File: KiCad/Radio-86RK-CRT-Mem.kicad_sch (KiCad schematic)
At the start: 20 parts, among them J1 Video, Q1 2N3904, U10 2716/КР573РФ5, U11 2716/КР573РФ5, U13 74198/К155ИР13, U15 7492/К155ИЕ4, U16 7486/К155ЛП5, U17 7474/К155ТМ2, U18 7408/К155ЛИ1, U19 7404/К155ЛН1, U8 8275/КР580ВГ75, U9 AS6C62256

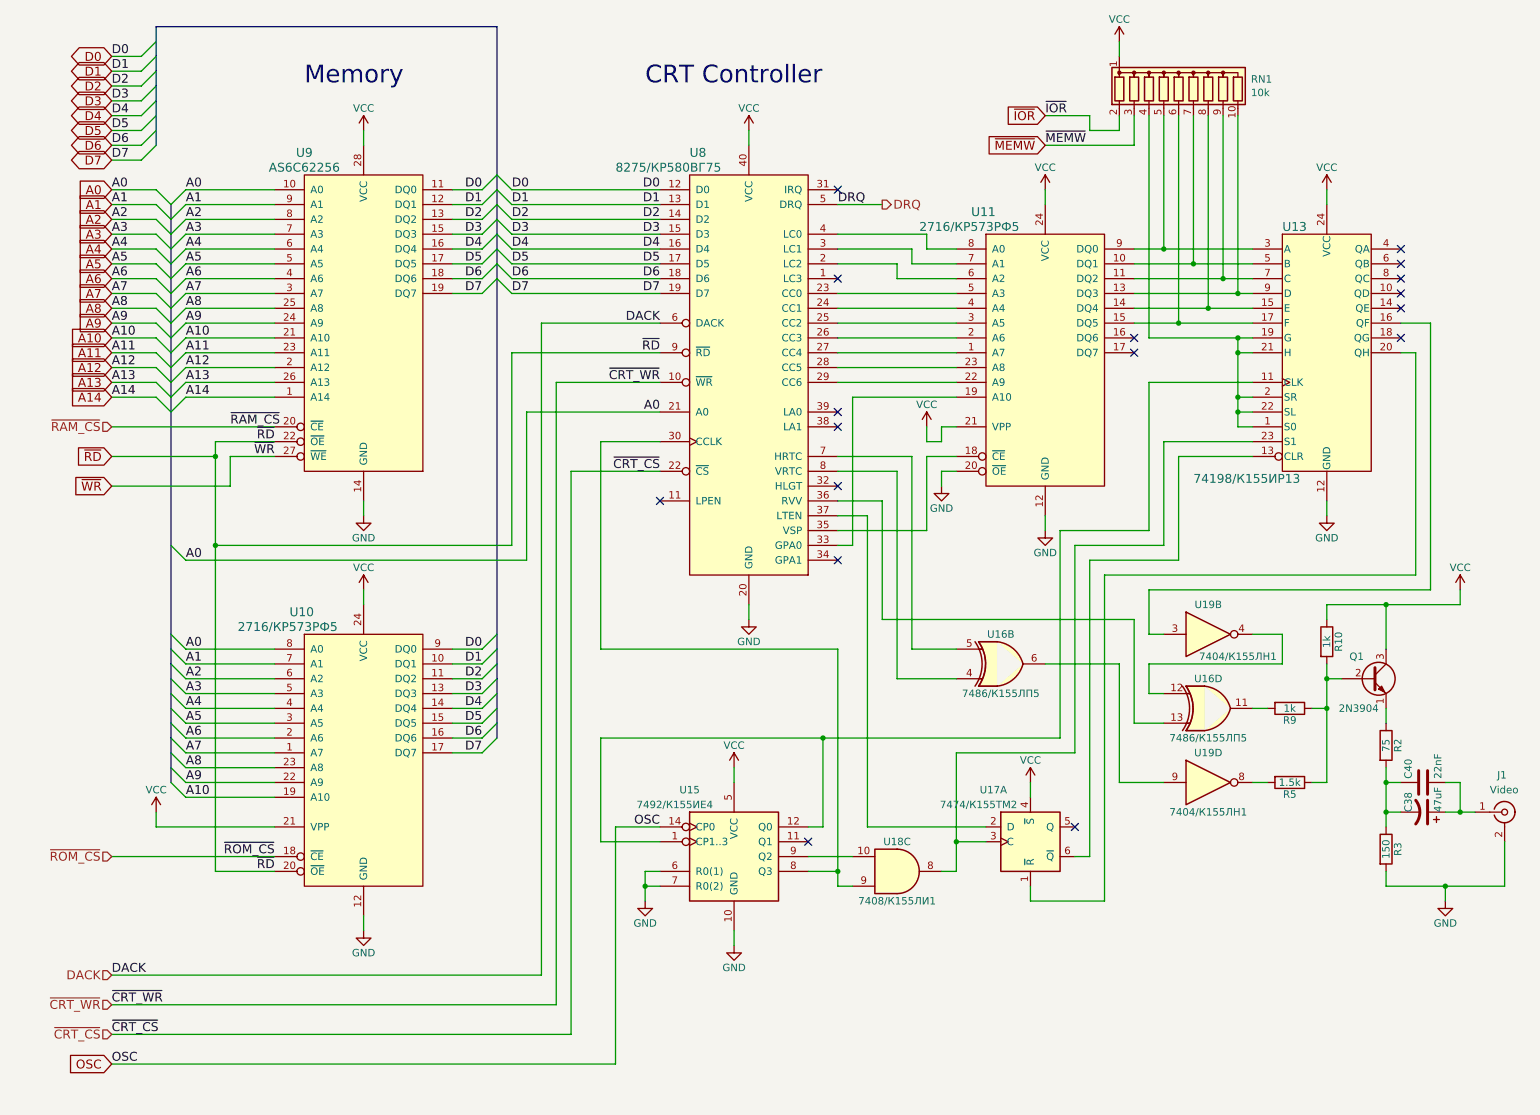
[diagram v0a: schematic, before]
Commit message: Add Version 1.4 files
Signed-off-by: Sergey Kiselev <skiselev@gmail.com>
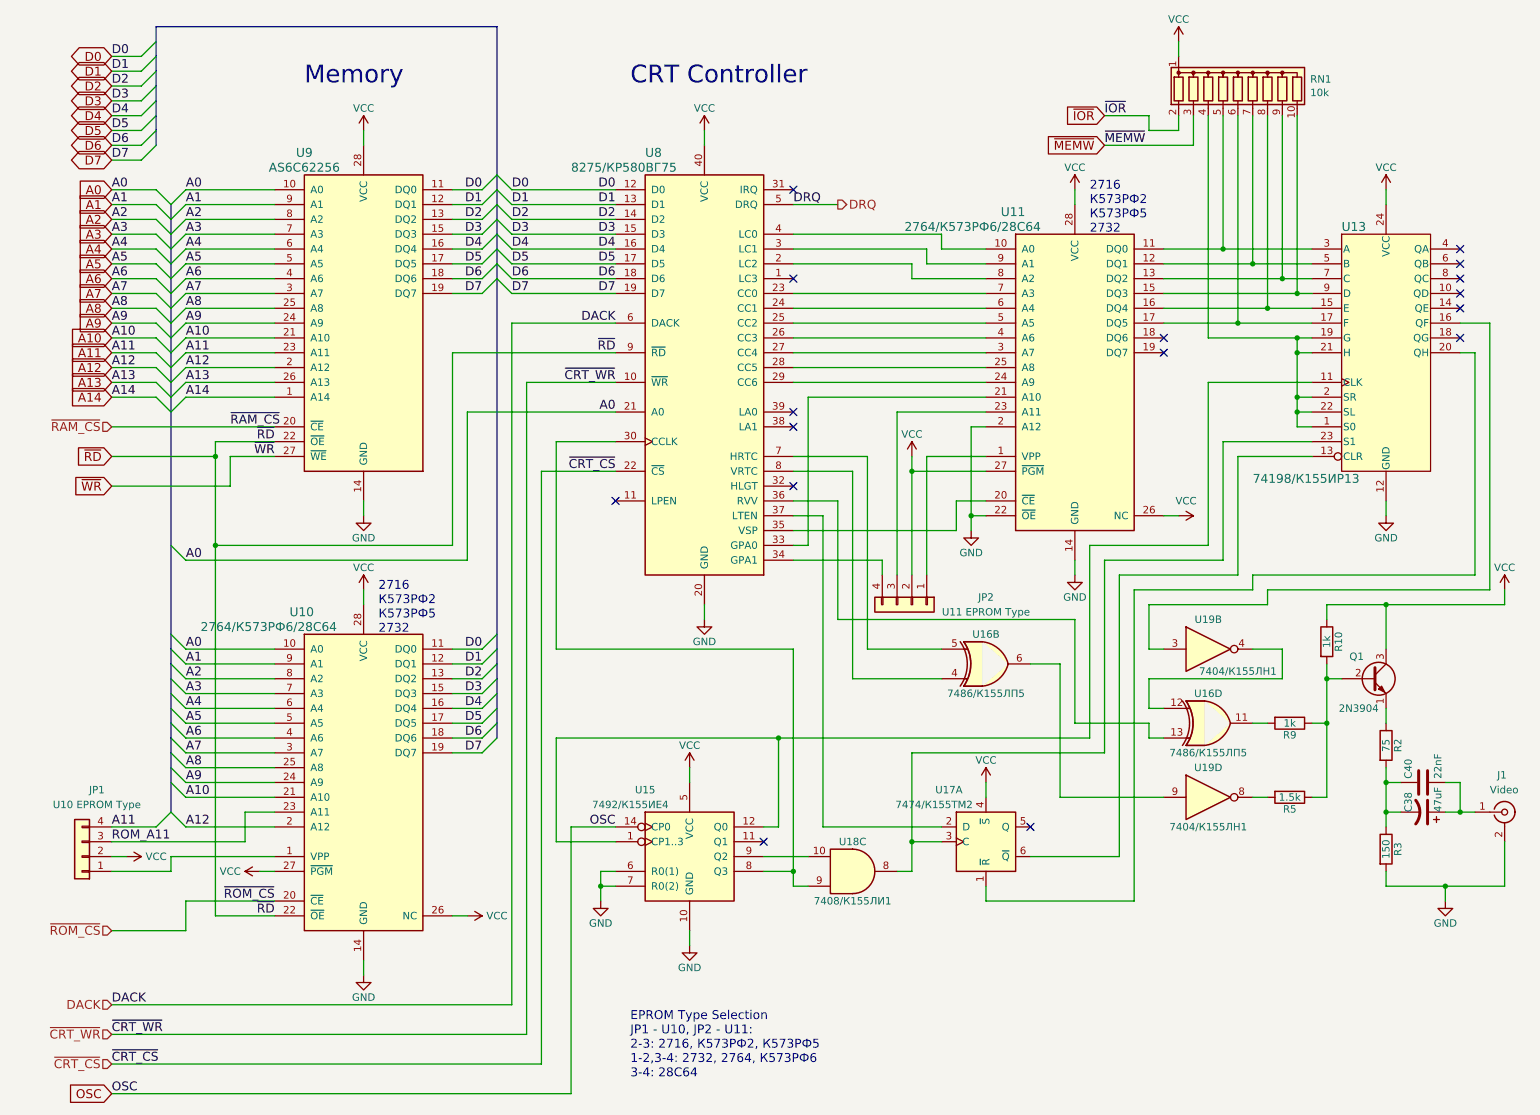
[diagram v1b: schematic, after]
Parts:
- removed U11: 2716/КР573РФ5, My_Components:IC_DIP24_600, symbol my_components:2716
- added JP1: U10 EPROM Type, My_Components:Conn_Pin_Header_4x1_2.54mm, symbol Connector_Generic:Conn_01x04
- added JP2: U11 EPROM Type, My_Components:Conn_Pin_Header_4x1_2.54mm, symbol Connector_Generic:Conn_01x04
- added U11: 2764/К573РФ6/28C64, My_Components:IC_DIP28_600, symbol my_components:27C64
- U10: value 2716/КР573РФ5 -> 2764/К573РФ6/28C64; footprint My_Components:IC_DIP24_600 -> My_Components:IC_DIP28_600; symbol my_components:2716 -> my_components:27C64
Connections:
- net A0: now also U10.10 (A0); no longer U10.8 (A0)
- net A1: now also U10.9 (A1); no longer U10.7 (A1)
- net A10: now also U10.21 (A10); no longer U10.19 (A10)
- net A11: now also JP1.4 (Pin_4)
- net A12: now also U10.2 (A12)
- net A2: now also U10.8 (A2); no longer U10.6 (A2)
- net A3: now also U10.7 (A3); no longer U10.5 (A3)
- net A4: now also U10.6 (A4); no longer U10.4 (A4)
- net A5: now also U10.5 (A5); no longer U10.3 (A5)
- net A6: now also U10.4 (A6); no longer U10.2 (A6)
- net A7: now also U10.3 (A7); no longer U10.1 (A7)
- net A8: now also U10.25 (A8); no longer U10.23 (A8)
- net A9: now also U10.24 (A9); no longer U10.22 (A9)
- net D0: now also U10.11 (DQ0); no longer U10.9 (DQ0)
- net D1: now also U10.12 (DQ1); no longer U10.10 (DQ1)
- net D2: now also U10.13 (DQ2); no longer U10.11 (DQ2)
- net D3: now also U10.15 (DQ3); no longer U10.13 (DQ3)
- net D4: now also U10.16 (DQ4); no longer U10.14 (DQ4)
- net D5: now also U10.17 (DQ5); no longer U10.15 (DQ5)
- net D6: now also U10.18 (DQ6); no longer U10.16 (DQ6)
- net D7: now also U10.19 (DQ7); no longer U10.17 (DQ7)
- net GND: now also U10.14 (GND), U11.14 (GND), U11.2 (A12), U11.22 (~{OE}); no longer U10.12 (GND)
- net VCC: now also U10.26 (NC), U10.27 (~{PGM}), U10.28 (VCC), JP1.2 (Pin_2), JP2.2 (Pin_2), U11.26 (NC), U11.27 (~{PGM}), U11.28 (VCC); no longer U10.21 (VPP), U10.24 (VCC)
- net ~{RD}: now also U10.22 (~{OE}); no longer U10.20 (~{OE})
- net ~{ROM_CS}: now also U10.20 (~{CE}); no longer U10.18 (~{CE})
- net at U8.27 (CC4): now also U11.3 (A7)
- net at RN1.7 (R6), U13.5 (B): now also U11.12 (DQ1)
- net at RN1.9 (R8), U13.7 (C): now also U11.13 (DQ2)
- net at RN1.10 (R9), U13.9 (D): now also U11.15 (DQ3)
- net at RN1.8 (R7), U13.15 (E): now also U11.16 (DQ4)
- net at RN1.6 (R5), U13.17 (F): now also U11.17 (DQ5)
- net at U8.35 (VSP): now also U11.20 (~{CE})
- net at U8.33 (GPA0): now also U11.21 (A10)
- net at U8.26 (CC3): now also U11.4 (A6)
- net at U8.29 (CC6): now also U11.24 (A9)
- net at U8.28 (CC5): now also U11.25 (A8)
- net at U8.25 (CC2): now also U11.5 (A5)
- net at U8.24 (CC1): now also U11.6 (A4)
- net at U8.23 (CC0): now also U11.7 (A3)
- net at U8.2 (LC2): now also U11.8 (A2)
- net at U8.3 (LC1): now also U11.9 (A1)
- net at U8.4 (LC0): now also U11.10 (A0)
- net at RN1.5 (R4), U13.3 (A): now also U11.11 (DQ0)
- net at U8.34 (GPA1): now also JP2.4 (Pin_4)
- new net: JP1.1 (Pin_1), U10.1 (VPP)
- new net: JP2.1 (Pin_1), U11.1 (VPP)
- new net: JP2.3 (Pin_3), U11.23 (A11)
- new net ROM_A11: JP1.3 (Pin_3), U10.23 (A11)
- no-connect marks 17 -> 16
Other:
- note added: "2716 К573РФ2 К573РФ5 2732"
- note added: "EPROM Type Selection JP1 - U10, JP2 - U11: 2-3: 2716, К573РФ2, К573РФ5 1-2,3-4: 2732, 2764, К573РФ6 3-4: 28C64"
- moved on the sheet: R5, R9, RN1, U13, U15, U16B, U16D, U17A, U18C, U19B, U19D
